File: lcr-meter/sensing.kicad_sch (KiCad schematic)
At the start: 4 parts, among them J4 Conn_01x04, U10 AD8216, U15 AD8216

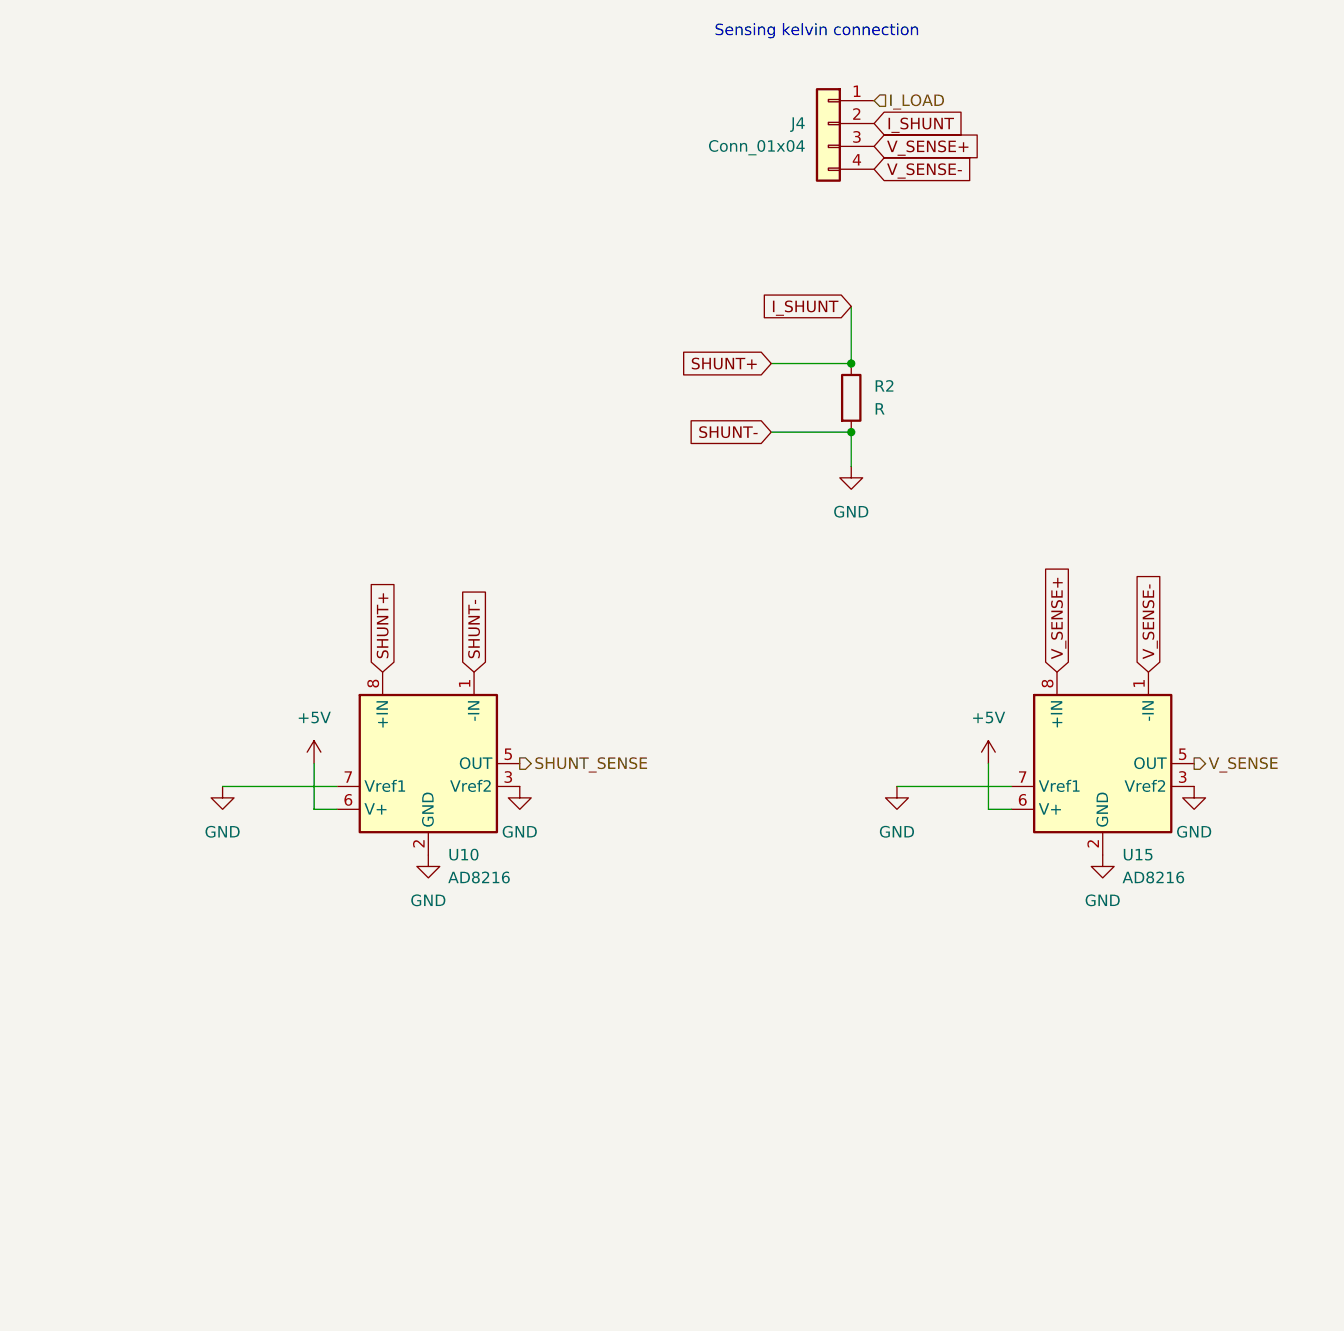
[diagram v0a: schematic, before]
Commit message: Breadboarding notes
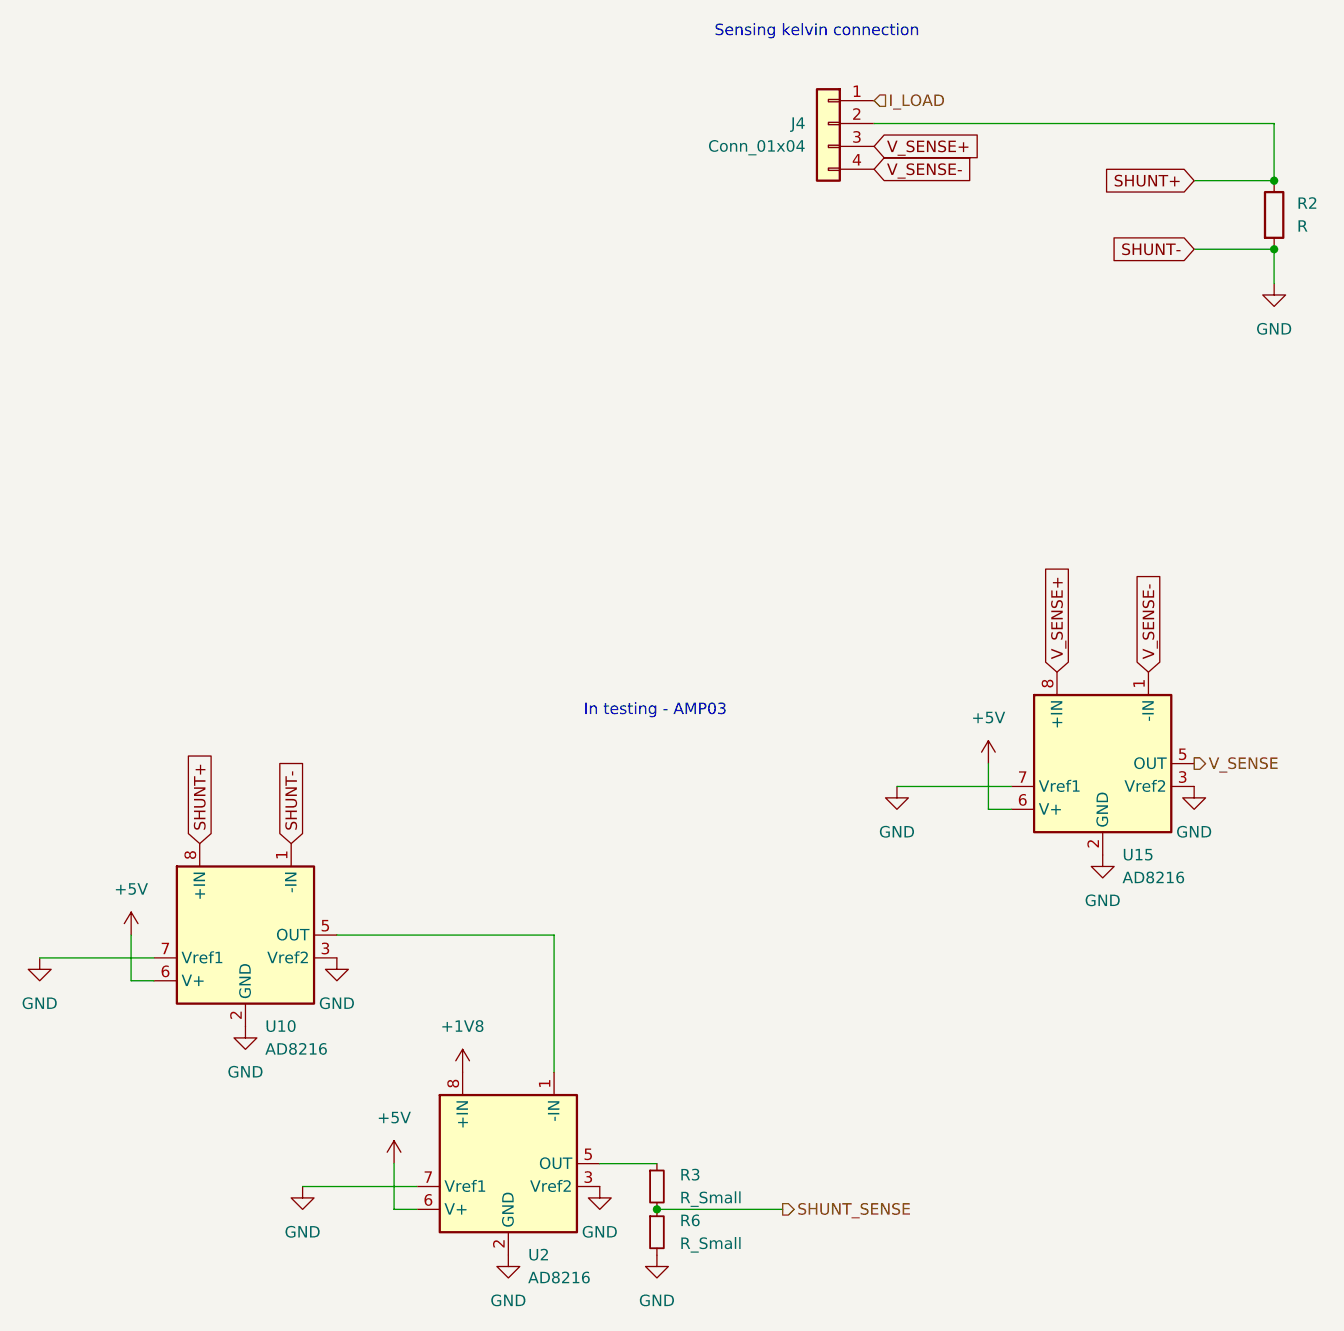
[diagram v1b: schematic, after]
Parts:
- added R3, R6: R_Small, symbol Device:R_Small
- added U2: AD8216, Package_SO:SOIC-8_3.9x4.9mm_P1.27mm, symbol Amplifier_Current:AD8216
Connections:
- net +5V: now also U2.6 (V+)
- net GND: now also R6.2, U2.2 (GND), U2.3 (Vref2), U2.7 (Vref1)
- net SHUNT_SENSE: now also R3.2, R6.1; no longer U10.5 (OUT)
- net I_SHUNT renamed SHUNT+
- new net: U10.5 (OUT), U2.1 (-IN)
- new net: R3.1, U2.5 (OUT)
- new net +1V8: U2.8 (+IN)
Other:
- note added: "In testing - AMP03"
- moved on the sheet: R2, U10
